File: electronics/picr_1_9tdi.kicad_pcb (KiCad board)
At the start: 4 copper layers, 50 x 50 mm, 84 parts, among them J1 10118193-0001LF, J2 Conn_01x02_Socket, J3 Conn_01x04_Pin, J4 Conn_01x03_Pin, J5 Conn_01x02_Pin, J6 Conn_01x03_Pin, J7 Conn_01x02_Socket, J8 Conn_01x02_Socket, J9 Conn_01x02_Socket, Q1 BUK6Y10-30PX, U1 DRV8243HQDGQRQ1, U10 215079-4, U11 215079-4, U12 SI8640AB-B-IS1, U13 SI8640AB-B-IS1, U14 MAX12930EASA+, U2 CM1223-02SO, U3 TPS62933, U4 DRV8243HQDGQRQ1, U5 MIC5504-3.3YM5, U6 DRV8243HQDGQRQ1, U7 STM32G441KBT6, U8 20021121-00010T4LF, U9 215079-4

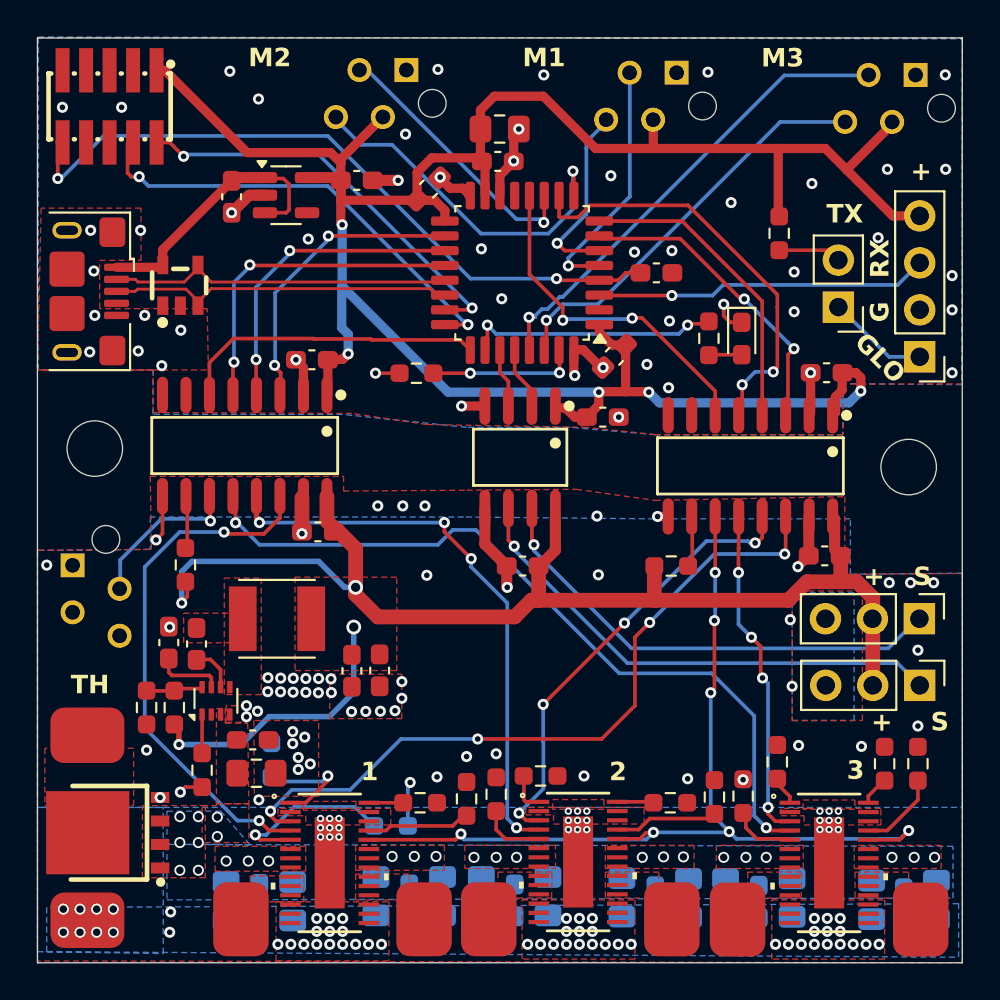
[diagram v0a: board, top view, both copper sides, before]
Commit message: .
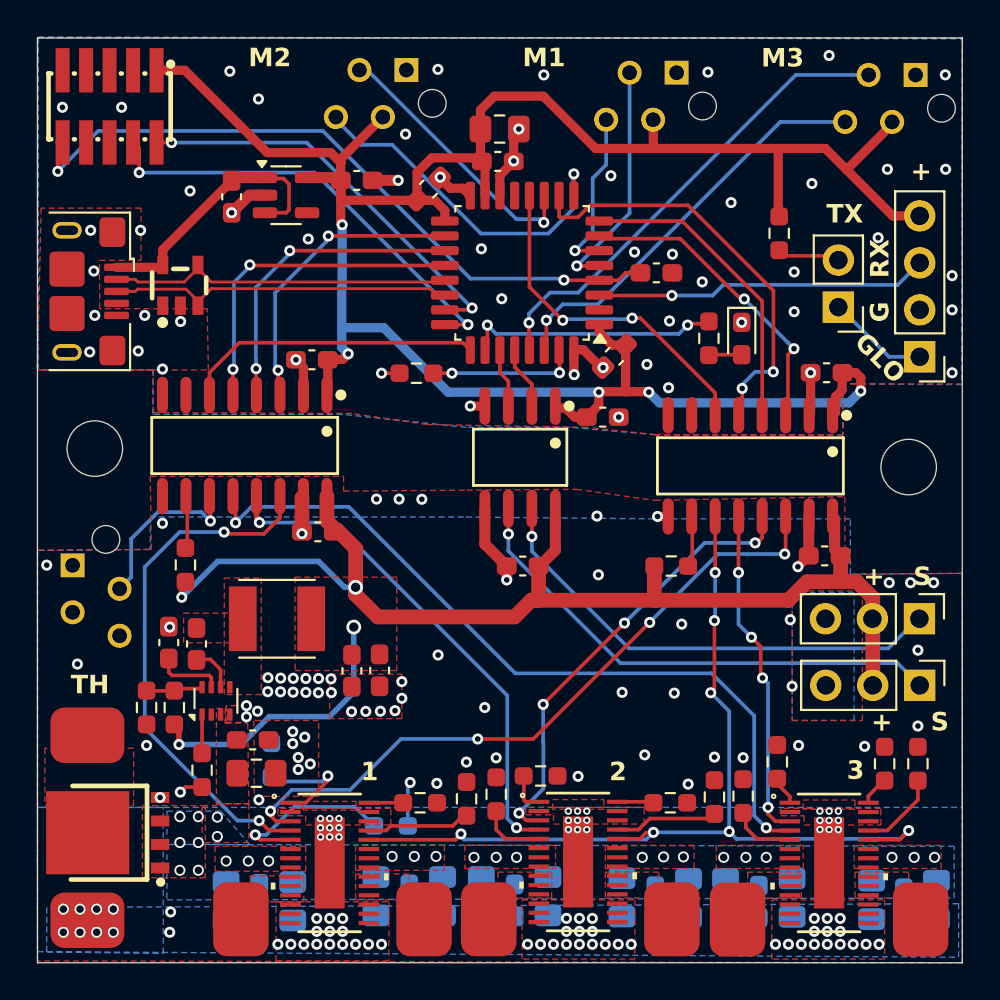
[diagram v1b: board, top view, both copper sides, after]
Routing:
- net /PWM_M2_O: track 31.6 -> 28.1 mm, vias 4 -> 2
- net GND_MOT: track 16.5 -> 13.6 mm, vias 142 -> 149
- net GND_MCU: track 23.0 -> 20.2 mm, vias 50 -> 53
- net /M1_DIR_O: track 39.3 -> 37.1 mm
- net /5V_MOT: track 79.5 -> 78.1 mm
- net /PWM_TH_O: track 7.80 -> 8.88 mm
- net /E_M1_B: track 10.1 -> 9.09 mm
- net +3.3V: track 127.6 -> 126.8 mm
- net /E_M1_A: track 13.4 -> 12.9 mm
- net /PWM_TH_I: track 16.6 -> 16.1 mm
- net /SWCLK: track 24.8 -> 24.3 mm
